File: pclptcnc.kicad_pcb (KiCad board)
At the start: 2 copper layers, 180.5 x 52.3 mm, 244 parts, among them P1 ARK825A-3, P3 ARK825A-4, P4 ARK825A-3, P5 ARK825A-3, P6 ARK825A-3, P7 ARK825A-3, P8 ARK825A-3, Q1 BC807-40, Q10 BC807-40, Q11 BC807-40, Q12 BC807-40, Q13 BC807-40, Q14 BC807-40, Q15 BC807-40, Q16 BC807-40, Q17 BC807-40, Q18 BC807-40, Q2 BC807-40, Q3 BC807-40, Q4 BC807-40, Q5 BC807-40, Q6 BC807-40, Q7 BC807-40, Q8 BC807-40, Q9 BC807-40, U1 74LVC1G3157GW, U10 SN74LVC2G17, U11 74HCT14, U12 SN74LVC2G17, U13 74HCT14, U2 HCPL2630, U3 HCPL2630, U4 HCPL2630, U5 HCPL2630, U6 HCPL2630, U7 HCPL2630, U8 74HCT14, U9 74HCT14, j1 DB25, j2 DB25

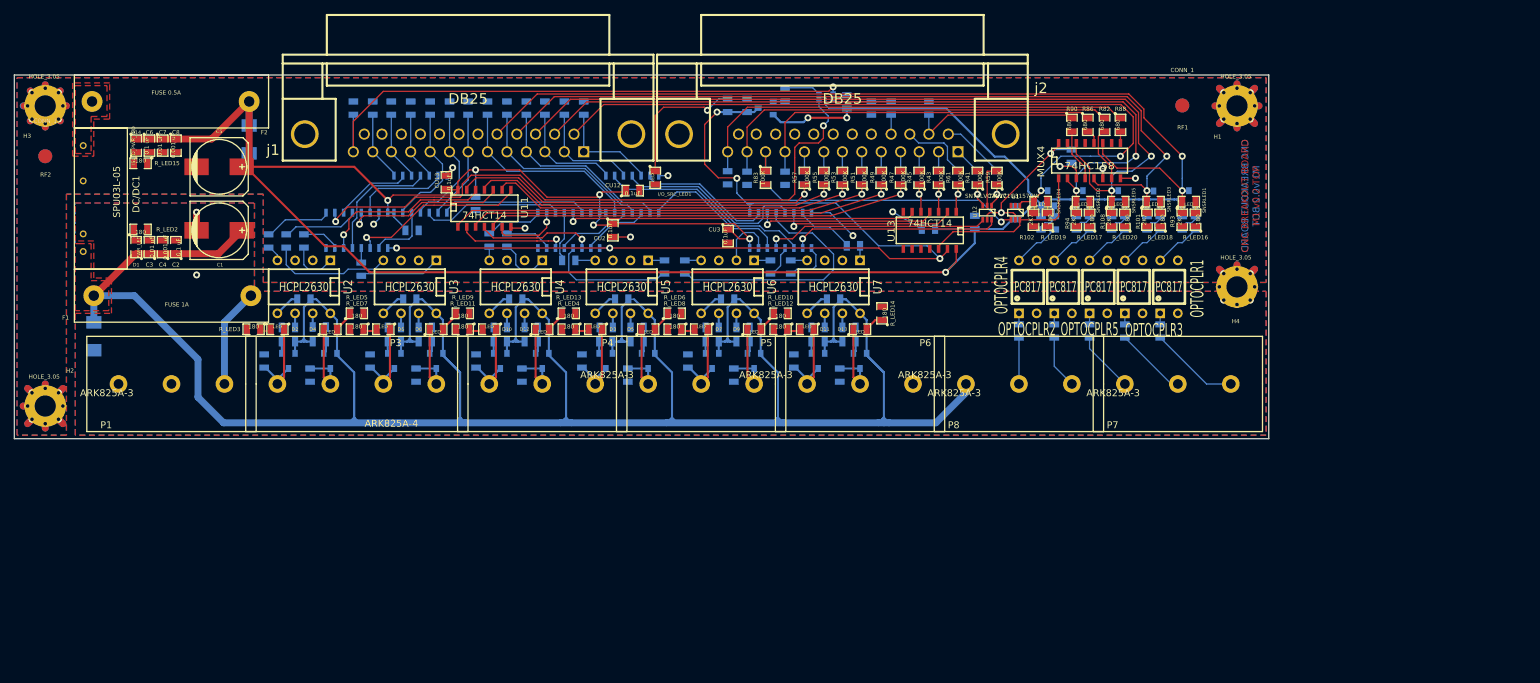
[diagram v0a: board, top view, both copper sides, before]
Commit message: revision b
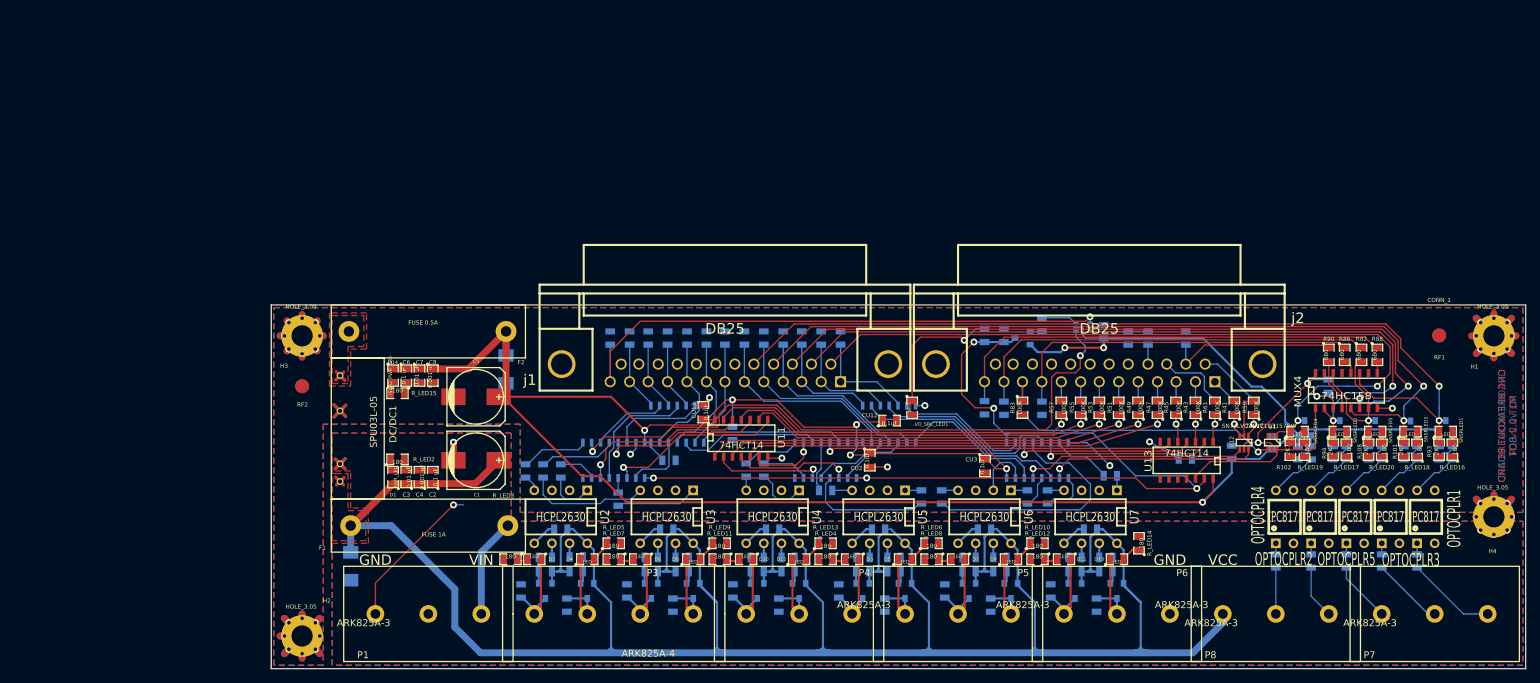
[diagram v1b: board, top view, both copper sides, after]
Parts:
- moved OPTOCPLR1 49.6 mm to (231.1, 108.6)
- moved OPTOCPLR5 49.6 mm to (220.9, 108.6)
- moved Q18 49.6 mm to (225.0, 92.1)
- moved R103 49.6 mm to (229.2, 95.6)
- moved R105 49.6 mm to (231.1, 95.6)
- moved R107 49.6 mm to (220.9, 111.2)
- moved R76 49.6 mm to (185.0, 117.5)
- moved R91 49.6 mm to (231.1, 111.2)
- moved R96 49.6 mm to (219.0, 95.6)
- moved R98 49.6 mm to (220.9, 95.6)
- moved SNSRLED5 49.6 mm to (225.0, 92.6)
- moved U12 49.6 mm to (206.2, 94.2)
- moved j2 49.6 mm to (185.4, 84.1)
- moved C5 49.6 mm to (95.7, 87.6)
- moved MUX4 49.6 mm to (220.9, 86.7)
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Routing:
- net /ISOLATED_GND: track 24.8 -> 55.5 mm, vias 1 -> 2
- net GND: track 388.7 -> 398.3 mm
- net /VCC_NFused: track 0.00 -> 3.41 mm
- net /ISOLATED_VCC: track 626.3 -> 629.4 mm
- net (no net): vias 1 -> 0
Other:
- board text added: "GND"
- board text added: "VCC"
- board text added: "VIN"
